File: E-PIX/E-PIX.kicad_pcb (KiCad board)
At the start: 6 copper layers, 40 x 40 mm, 47 parts, among them J1 USB_C_Receptacle_USB2.0, J2 BNO055, J3 ADC, J4 ADC, Q1 BSS138, Q2 BSS138, SW1 SW, SW2 SW_Push, U1 Conn_03x04, U2 Conn_03x04, U3 TC7WH241FK, U4 TC7WH241FK, U5 NJM7805SDL1, U6 AZ1117-3.3, U7 ESP32-C3-WROOM-02, U8 BTS6142D

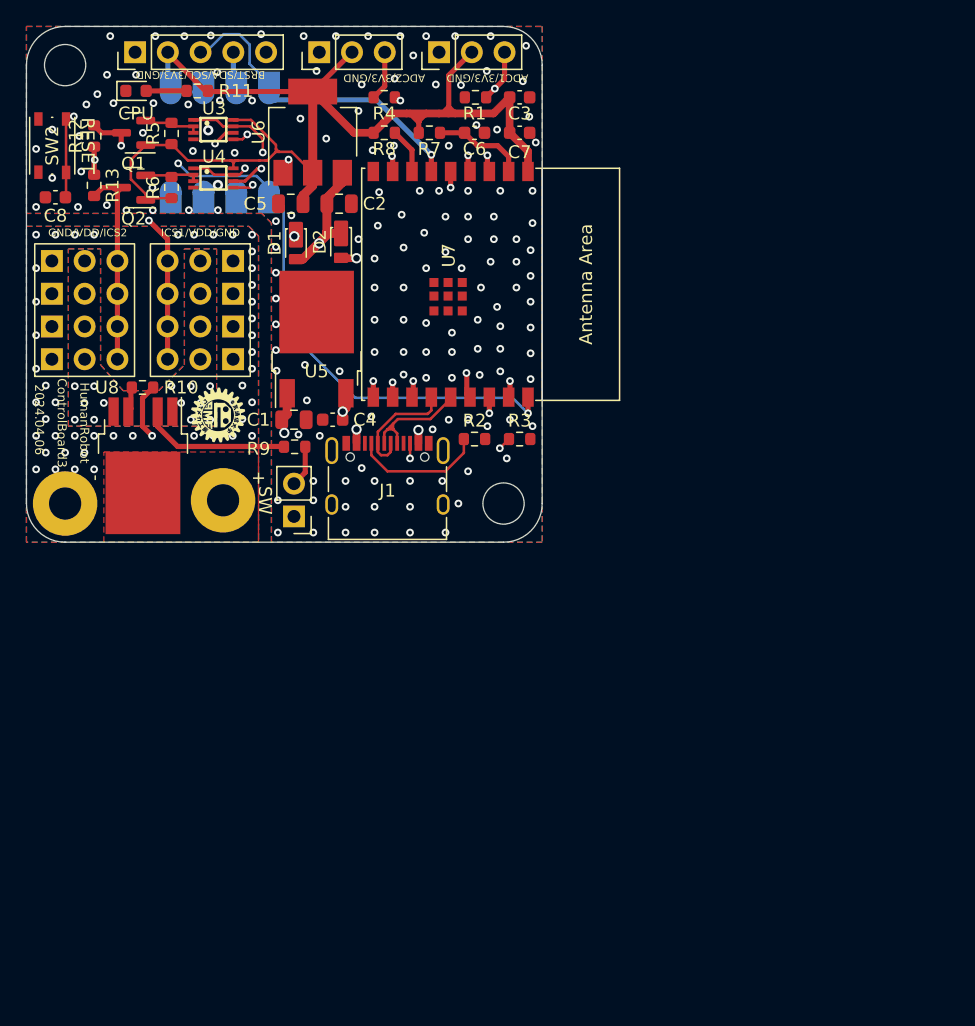
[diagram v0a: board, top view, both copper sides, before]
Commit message: finish eeschema. start placing tips
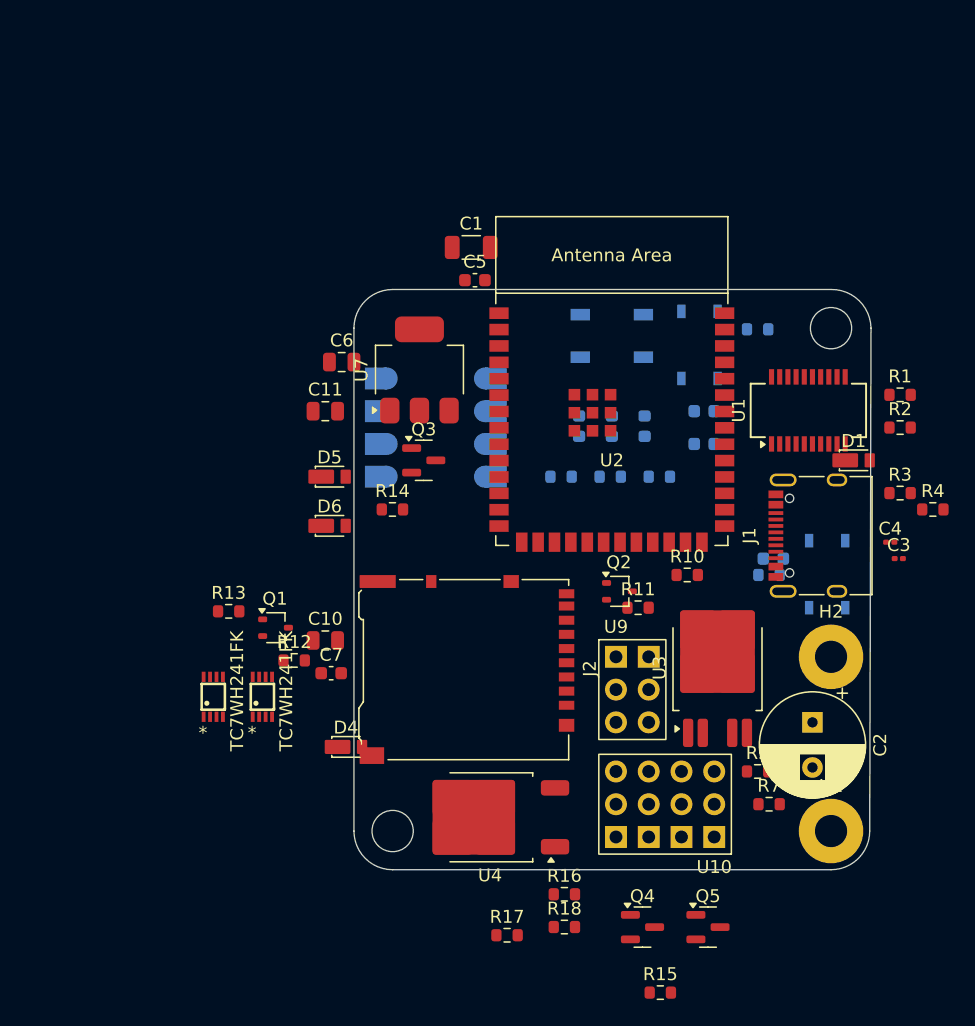
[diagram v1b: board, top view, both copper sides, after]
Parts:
- removed G***: LOGO, Logo:Robo
- removed G***: LOGO, Logo:L6
- removed J3, J4: ADC, Connector_PinHeader_2.54mm:PinHeader_1x03_P2.54mm_Vertical
- added C10: 10u/50V/2012, Capacitor_SMD:C_0805_2012Metric, F.Cu at (123.2, 107.6)
- added C11: 22u/25V/2012, Capacitor_SMD:C_0805_2012Metric, F.Cu at (123.2, 89.8)
- added C12: 0.1u/25V, Capacitor_SMD:C_0603_1608Metric, B.Cu at (157.9, 101.3)
- added C9: 0.1u/25V, Capacitor_SMD:C_0603_1608Metric, B.Cu at (152.6, 89.8)
- added D4: CUHS20S60/2A/60V, Diode:Diode_US2H, F.Cu at (124.8, 115.9)
- added D5: CUHS20S60/2A/60V, Diode:Diode_US2H, F.Cu at (123.5, 94.9)
- added D6: CUHS20S60/2A/60V, Diode:Diode_US2H, F.Cu at (123.5, 98.7)
- added D7: LED, LED_SMD:LED_0603_1608Metric, B.Cu at (142.9, 91.0)
- added D8: WS2812B, LED_SMD:LED_WS2812B_PLCC4_5.0x5.0mm_P3.2mm, B.Cu at (145.4, 84.0)
- added Q3: AO3401A, Package_TO_SOT_SMD:SOT-23, F.Cu at (130.8, 93.7)
- added Q4: BSS138, Package_TO_SOT_SMD:SOT-23, F.Cu at (147.8, 129.8)
- added Q5: BSS138, Package_TO_SOT_SMD:SOT-23, F.Cu at (152.9, 129.8)
- added R14: 4.7, Resistor_SMD:R_0603_1608Metric, F.Cu at (128.4, 97.5)
- added R15: 2.2k, Resistor_SMD:R_0603_1608Metric, F.Cu at (149.2, 134.9)
- added R16: 2.2k, Resistor_SMD:R_0603_1608Metric, F.Cu at (141.7, 127.3)
- added R17: 2.2k, Resistor_SMD:R_0603_1608Metric, F.Cu at (137.3, 130.5)
- added R18: 2.2k, Resistor_SMD:R_0603_1608Metric, F.Cu at (141.7, 129.8)
- added R19: 10k, Resistor_SMD:R_0603_1608Metric, B.Cu at (157.6, 102.5)
- added R20: 100, Resistor_SMD:R_0603_1608Metric, B.Cu at (141.5, 94.9)
- added U10: Conn_03x04, Conn:PinHeader_03x04_P2.54mm_Vertical, F.Cu at (153.3, 122.9)
- C1: value 1u/50V/2012 -> 10u/35V; footprint Capacitor_SMD:C_0805_2012Metric -> Capacitor_SMD:C_1206_3216Metric
- C2: value 10u/50V/2012 -> C_Polarized; footprint Capacitor_SMD:C_0805_2012Metric -> Capacitor_THT:CP_Radial_D8.0mm_P3.50mm
- C3: value 10u/35V -> 47p; footprint Capacitor_SMD:C_0603_1608Metric -> Capacitor_SMD:C_0201_0603Metric
- C4: value 0.1u/25V -> 47p; footprint Capacitor_SMD:C_0603_1608Metric -> Capacitor_SMD:C_0201_0603Metric
- C5: value 22u/25V/2012 -> 0.1u/25V; footprint Capacitor_SMD:C_0805_2012Metric -> Capacitor_SMD:C_0603_1608Metric
- C6: value 1u/16V -> 1u/50V/2012; footprint Capacitor_SMD:C_0603_1608Metric -> Capacitor_SMD:C_0805_2012Metric
- C8, R9: moved to B.Cu
- D2: value CUHS20S60/2A/60V -> LED; footprint Diode:Diode_US2H -> LED_SMD:LED_0603_1608Metric; moved to B.Cu
- D3: value GREEN -> LED; moved to B.Cu
- J1: footprint Connector_USB:USB_C_Receptacle_XKB_U262-16XN-4BVC11 -> Connector_USB:USB_C_Receptacle_XKB_U262-16XN-4BVC11_with_model
- J2: value BNO055 -> DM3AT-SF-PEJM5; footprint Connector_PinHeader_2.54mm:PinHeader_1x05_P2.54mm_Vertical -> Connector_Card:microSD_HC_Hirose_DM3AT-SF-PEJM5
- Q1, Q2: value BSS138 -> 2SC4213; footprint Package_TO_SOT_SMD:SOT-23 -> Package_TO_SOT_SMD:SOT-323_SC-70
- R1: value 10k -> 5.1k
- R10: value 10k -> 47k
- R11: value 510 -> 47k
- R12, R13: value 2.2k -> 470k
- R3: value 5.1k -> 27
- R4: value 10k -> 27
- R5: value 2.2k -> 10k
- R6: value 2.2k -> 100; moved to B.Cu
- R8: value 10k -> 100; moved to B.Cu
- SW1: value SW -> SW_Push; footprint Connector_PinHeader_2.54mm:PinHeader_1x02_P2.54mm_Vertical -> Button_Switch_SMD:SKRPACE010; moved to B.Cu
- SW2: footprint Button_Switch_SMD:SW_Push_1P1T_NO_Vertical_Wuerth_434133025816 -> Button_Switch_SMD:SKRPACE010; moved to B.Cu
- U1: value Conn_03x04 -> FT231XS; footprint Conn:PinHeader_03x04_P2.54mm_Vertical -> Package_SO:SSOP-20_3.9x8.7mm_P0.635mm
- U2: value Conn_03x04 -> ESP32-S3-WROOM-1; footprint Conn:PinHeader_03x04_P2.54mm_Vertical -> Espressif:ESP32-S3-WROOM-1
- U3: value TC7WH241FK -> BTS6142D; footprint Logic:US-8 -> Package_TO_SOT_SMD:TO-252-4
- U4: value TC7WH241FK -> NJM7805SDL1; footprint Logic:US-8 -> Package_TO_SOT_SMD:TO-252-2
- U5: value NJM7805SDL1 -> TC7WH241FK; footprint Package_TO_SOT_SMD:TO-252-2 -> Logic:US-8
- U6: value AZ1117-3.3 -> TC7WH241FK; footprint Package_TO_SOT_SMD:SOT-223-3_TabPin2 -> Logic:US-8
- U7: value ESP32-C3-WROOM-02 -> AZ1117-3.3; footprint Espressif:ESP32-C3-WROOM-02 -> Package_TO_SOT_SMD:SOT-223-3_TabPin2
- U8: value BTS6142D -> ~; footprint Package_TO_SOT_SMD:TO-252-4 -> IMU:BNO055; moved to B.Cu
- U9: value ~ -> Conn_03x02; footprint IMU:BNO055 -> Conn:PinHeader_03x02_P2.54mm_Vertical; moved to F.Cu
- moved SW2 68.7 mm to (162.1, 102.5), turned to 90 degrees
- moved R5 67.2 mm to (156.7, 117.8), turned to 0 degrees
- moved H1 64.6 mm to (162.4, 122.4)
- moved H4 64.6 mm to (128.4, 122.4)
- moved R7 58.4 mm to (157.6, 120.3)
- moved U3 57.2 mm to (153.6, 109.7), turned to 90 degrees
- moved C2 54.5 mm to (161.0, 114.0), turned to -90 degrees
- moved J2 54.4 mm to (134.2, 109.9), turned to -90 degrees
- moved U4 54.0 mm to (136.0, 121.3), turned to 180 degrees
- moved C8 53.8 mm to (152.6, 92.4)
- moved R4 53.2 mm to (170.3, 97.5), turned to 0 degrees
- moved R11 52.7 mm to (147.4, 105.1), turned to 0 degrees
- moved U9 50.3 mm to (145.7, 108.9), turned to 0 degrees
- moved Q2 49.0 mm to (146.0, 103.8), turned to 0 degrees
- moved H2 48.7 mm to (162.4, 108.9)
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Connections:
- C1 pad 2: VDD -> +3V3
- C2 pad 1: GND -> VDD
- C2 pad 2: +5V -> GND
- C3 pad 1: +3V3 -> GND
- C3 pad 2: GND -> Net-(U1-USBDM)
- C4 pad 1: +5V -> GND
- C4 pad 2: GND -> Net-(U1-USBDP)
- C5 pad 1: +3V3 -> GND
- C5 pad 2: GND -> +3V3
- C6 pad 1: Net-(U7-EN/CHIP_PU) -> GND
- C6 pad 2: GND -> VSS
- C7 pad 1: +3V3 -> +5V
- C8 pad 1: /RST -> /EN
- D1 pad 1: VDD -> +5V
- D1 pad 2: +5V -> Net-(D1-A)
- D2 pad 1: +5V -> Net-(D2-K)
- D2 pad 2: Net-(D2-A) -> VSS
- D3 pad 1: GND -> Net-(D3-K)
- D3 pad 2: Net-(D3-A) -> +3V3
- J1 pad A4: Net-(D2-A) -> Net-(D1-A)
- J1 pad A9: Net-(D2-A) -> Net-(D1-A)
- J1 pad B4: Net-(D2-A) -> Net-(D1-A)
- J1 pad B9: Net-(D2-A) -> Net-(D1-A)
- J1 pad S1: unconnected-(J1-SHIELD-PadS1) -> GND
- J2 pad 1: GND -> unconnected-(J2-DAT2-Pad1)
- J2 pad 2: +3V3 -> /CS
- J2 pad 3: /SCL -> /MOSI
- J2 pad 4: /SDA -> +3V3
- J2 pad 5: /BNO055RST -> /CLK
- Q1 pad 1: +3V3 -> Net-(Q1-B)
- Q1 pad 2: /ICS1_3V3 -> /RTS
- Q1 pad 3: /ICS1_5V -> /EN
- Q2 pad 1: +3V3 -> Net-(Q2-B)
- Q2 pad 2: /ICS2_3V3 -> /DTR
- Q2 pad 3: /ICS2_5V -> /BOOT
- R1 pad 1: GND -> Net-(J1-CC1)
- R1 pad 2: /ADC1 -> GND
- R10 pad 1: Net-(U8-IS) -> Net-(Q1-B)
- R10 pad 2: GND -> /DTR
- R11 pad 1: +3V3 -> Net-(Q2-B)
- R11 pad 2: Net-(D3-A) -> /RTS
- R12 pad 1: +5V -> GND
- R12 pad 2: /ICS1_5V -> /DTR
- R13 pad 1: +5V -> GND
- R13 pad 2: /ICS2_5V -> /RTS
- R2 pad 1: Net-(J1-CC1) -> Net-(J1-CC2)
- R3 pad 1: Net-(J1-CC2) -> /D-
- R3 pad 2: GND -> Net-(U1-USBDM)
- R4 pad 1: GND -> Net-(U1-USBDP)
- R4 pad 2: /ADC2 -> /D+
- R5 pad 1: +3V3 -> Net-(U3-IN)
- R5 pad 2: /ICS1_3V3 -> /EN_Power
- R6 pad 1: +3V3 -> Net-(D2-K)
- R6 pad 2: /ICS2_3V3 -> GND
- R7 pad 1: +3V3 -> Net-(U3-IS)
- R7 pad 2: Net-(U7-EN/CHIP_PU) -> GND
- R8 pad 1: +3V3 -> Net-(D3-K)
- R8 pad 2: Net-(U7-GPIO8) -> GND
- R9 pad 1: Net-(SW1A-B) -> /EN
- R9 pad 2: Net-(U8-IN) -> +3V3
- SW1 pad 1: GND -> /EN
- SW1 pad 2: Net-(SW1A-B) -> GND
- SW2 pad 1: /RST -> /SW
- U1 pad 1: GND -> /DTR
- U1 pad 2: VSS -> /RTS
- U1 pad 3: /ICS1_5V -> +3V3
- U2 pad 2: VSS -> +3V3
- U2 pad 3: /ICS2_5V -> /EN
- U3 pad 1: /EN1 -> VSS
- U3 pad 2: /ICS1_3V3 -> Net-(U3-IN)
- U3 pad 3: /ICS1_3V3 -> VDD
- U3 pad 4: GND -> Net-(U3-IS)
- U3 pad 5: /TX1 -> VSS
- U4 pad 1: /EN2 -> VSS
- U4 pad 2: /ICS2_3V3 -> GND
- U4 pad 3: /ICS2_3V3 -> +5V
- U5 pad 1: VDD -> /EN1
- U5 pad 2: GND -> /ICS1_3V3
- U5 pad 3: +5V -> /ICS1_3V3
- U6 pad 1: GND -> /EN2
- U6 pad 2: +3V3 -> /ICS2_3V3
- U6 pad 3: +5V -> /ICS2_3V3
- U7 pad 1: +3V3 -> GND
- U7 pad 2: Net-(U7-EN/CHIP_PU) -> +3V3
- U7 pad 3: /ADC1 -> VSS
- U8 pad 1: VSS -> +3V3
- U8 pad 2: Net-(U8-IN) -> GND
- U8 pad 3: VDD -> /SDA
- U8 pad 4: Net-(U8-IS) -> /SCL
- U8 pad 5: VSS -> /BNO_RST
- U9 pad 1: +3V3 -> GND
- U9 pad 2: GND -> VSS
- U9 pad 3: /SDA -> /ICS1_5V
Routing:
- net +3V3: track 93.1 -> 0.00 mm
- net /BNO055RST: track 57.5 -> 0.00 mm, vias 2 -> 0
- net +5V: track 48.6 -> 0.00 mm, vias 3 -> 0
- net /EN2: track 39.6 -> 0.00 mm, vias 2 -> 0
- net /RST: track 33.9 -> 0.00 mm, vias 2 -> 0
- net /RX2: track 33.8 -> 0.00 mm, vias 2 -> 0
- net /RX1: track 31.4 -> 0.00 mm, vias 2 -> 0
- net /TX1: track 31.3 -> 0.00 mm, vias 2 -> 0
- net /EN1: track 29.6 -> 0.00 mm, vias 2 -> 0
- net /TX2: track 28.2 -> 0.00 mm, vias 2 -> 0
- net /SDA: track 25.9 -> 0.00 mm, vias 1 -> 0
- net VDD: track 25.7 -> 0.00 mm, vias 2 -> 0
- net /SCL: track 25.0 -> 0.00 mm, vias 1 -> 0
- net Net-(D2-A): track 21.5 -> 0.00 mm, vias 3 -> 0
- net /ICS1_5V: track 21.2 -> 0.00 mm, vias 2 -> 0
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- removed copper zone on B.Cu, net GND
- removed copper zone on F.Cu, net GND
- removed copper zone on In1.Cu, net GND
- removed copper zone on In2.Cu, net GND
- removed copper zone on In3.Cu, net GND
- removed copper zone on In4.Cu, net GND
- removed copper zone on F.Cu, net VDD
- removed copper zone on B.Cu, net VSS
- removed copper zone on F.Cu, net VSS
- removed copper zone on In1.Cu, net VSS
- removed copper zone on In2.Cu, net VSS
- removed copper zone on In3.Cu, net VSS
- removed copper zone on In4.Cu, net VSS
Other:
- board size 40 x 40 mm -> 40.1 x 45 mm
- copper layers 6 -> 2
- board text removed: "+"
- board text removed: "-"
- board text removed: "2024.04.06"
- board text removed: "ADC1/3V3/GND"
- board text removed: "ADC2/3V3/GND"
- board text removed: "AE-BNO055-BO"
- board text removed: "BRST/SDA/SCL/3V3/GND"
- board text removed: "CPU"
- board text removed: "ControlBoard3"
- board text removed: "GND/VDD/ICS2"
- board text removed: "HumanRobot"
- board text removed: "ICS1/VDD/GND"
- board text removed: "RESET"
- board text removed: "SW"
- board text removed: "VIN"
